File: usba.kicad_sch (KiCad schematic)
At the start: 8 parts, among them J8 Conn_01x06_Pin, J9 Conn_01x06_Pin, U4 PUSB3FR4-ES, U5 XDUF-0426-081_C18202150, U6 RH792A

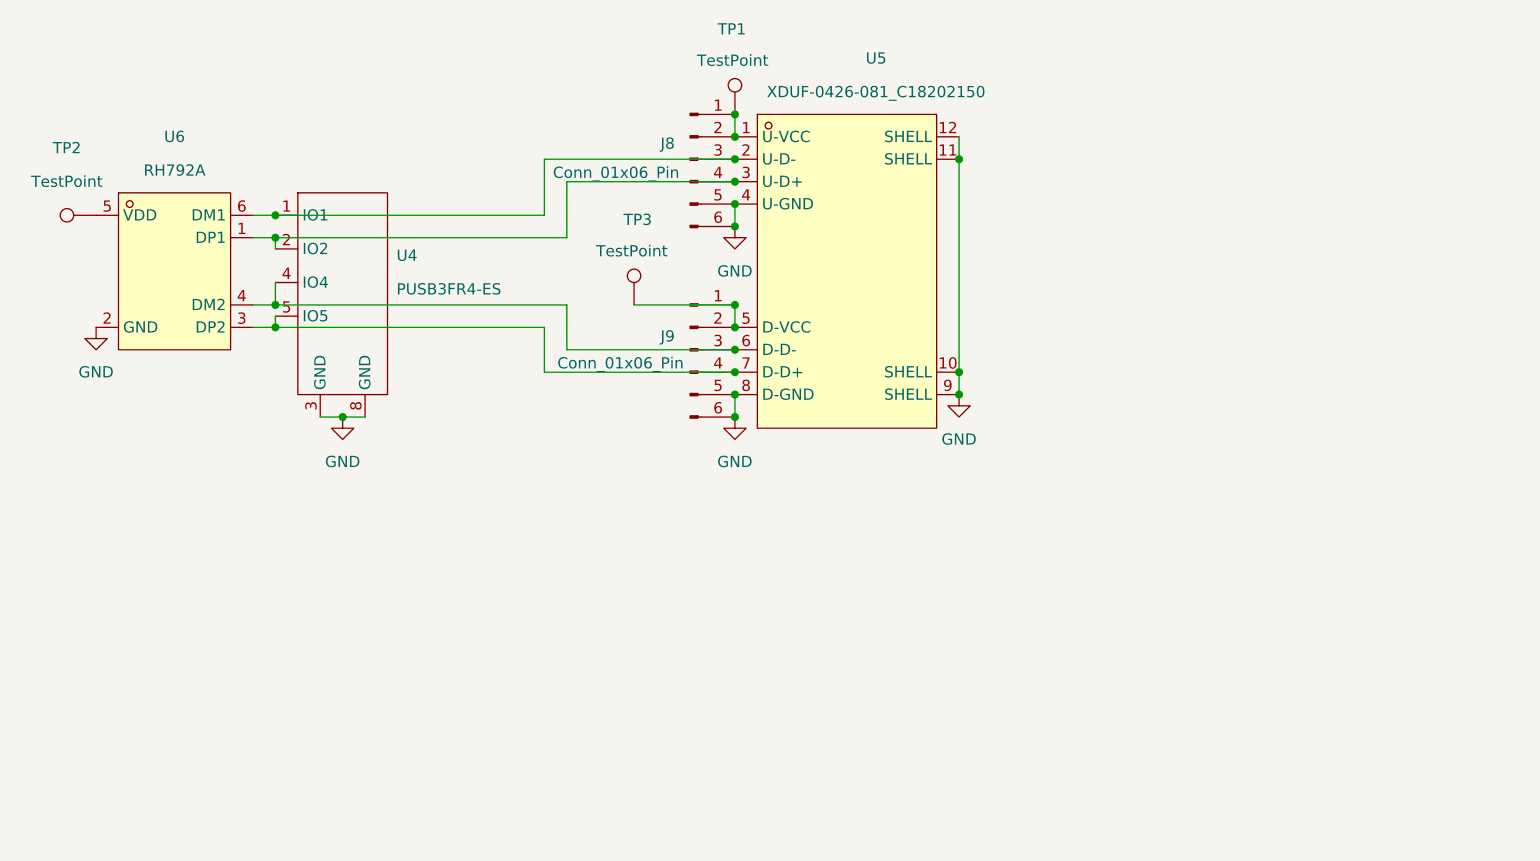
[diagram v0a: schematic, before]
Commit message: no more modules, its gonna work first try :fire: i love infineon and their ICs so much
Signed-off-by: Toby Cm <toby@vsus.app>
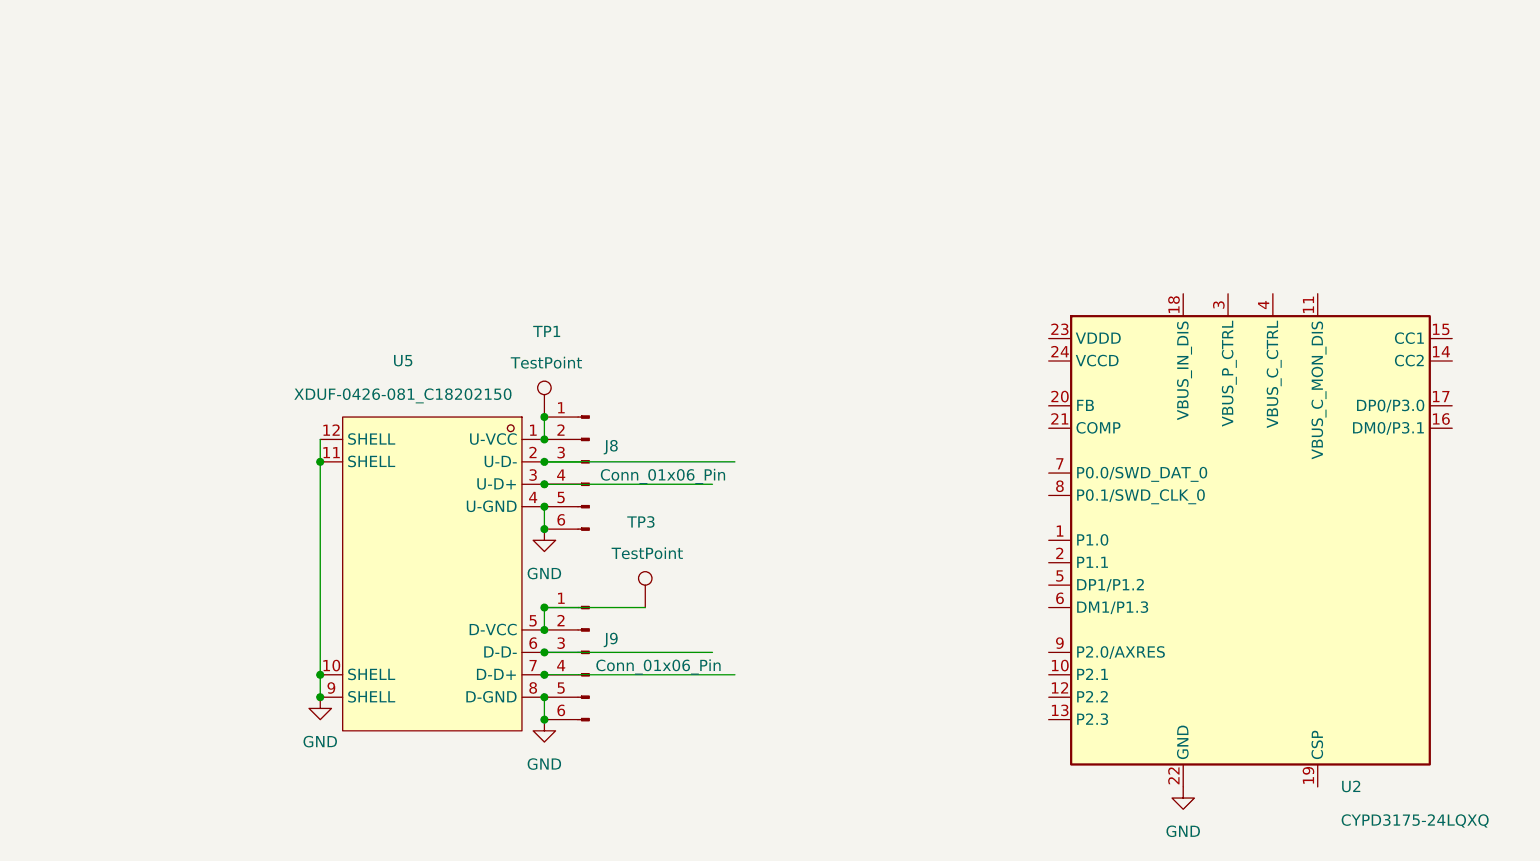
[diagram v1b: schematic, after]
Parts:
- removed TP2: TestPoint, TestPoint:TestPoint_Pad_D2.0mm, symbol Connector:TestPoint
- removed U4: PUSB3FR4-ES, Package_DFN_QFN:Diodes_UDFN-10_1.0x2.5mm_P0.5mm, symbol ElecSuper:PUSB3FR4-ES
- removed U6: RH792A, easyeda2kicad:SOT-23-6_L2.9-W1.6-P0.95-LS2.9-BL, symbol easyeda2kicad:RH792A
- added U2: CYPD3175-24LQXQ, Package_DFN_QFN:QFN-24-1EP_4x4mm_P0.5mm_EP2.75x2.75mm, symbol Interface_USB:CYPD3175-24LQXQ
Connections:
- net GND: now also U2.22 (GND), U2.25 (GND)
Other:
- moved on the sheet: J8, J9, TP1, TP3, U5
